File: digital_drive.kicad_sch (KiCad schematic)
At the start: 19 parts, among them U1501 EPC23104ENGRT, U1502 EPC23104ENGRT

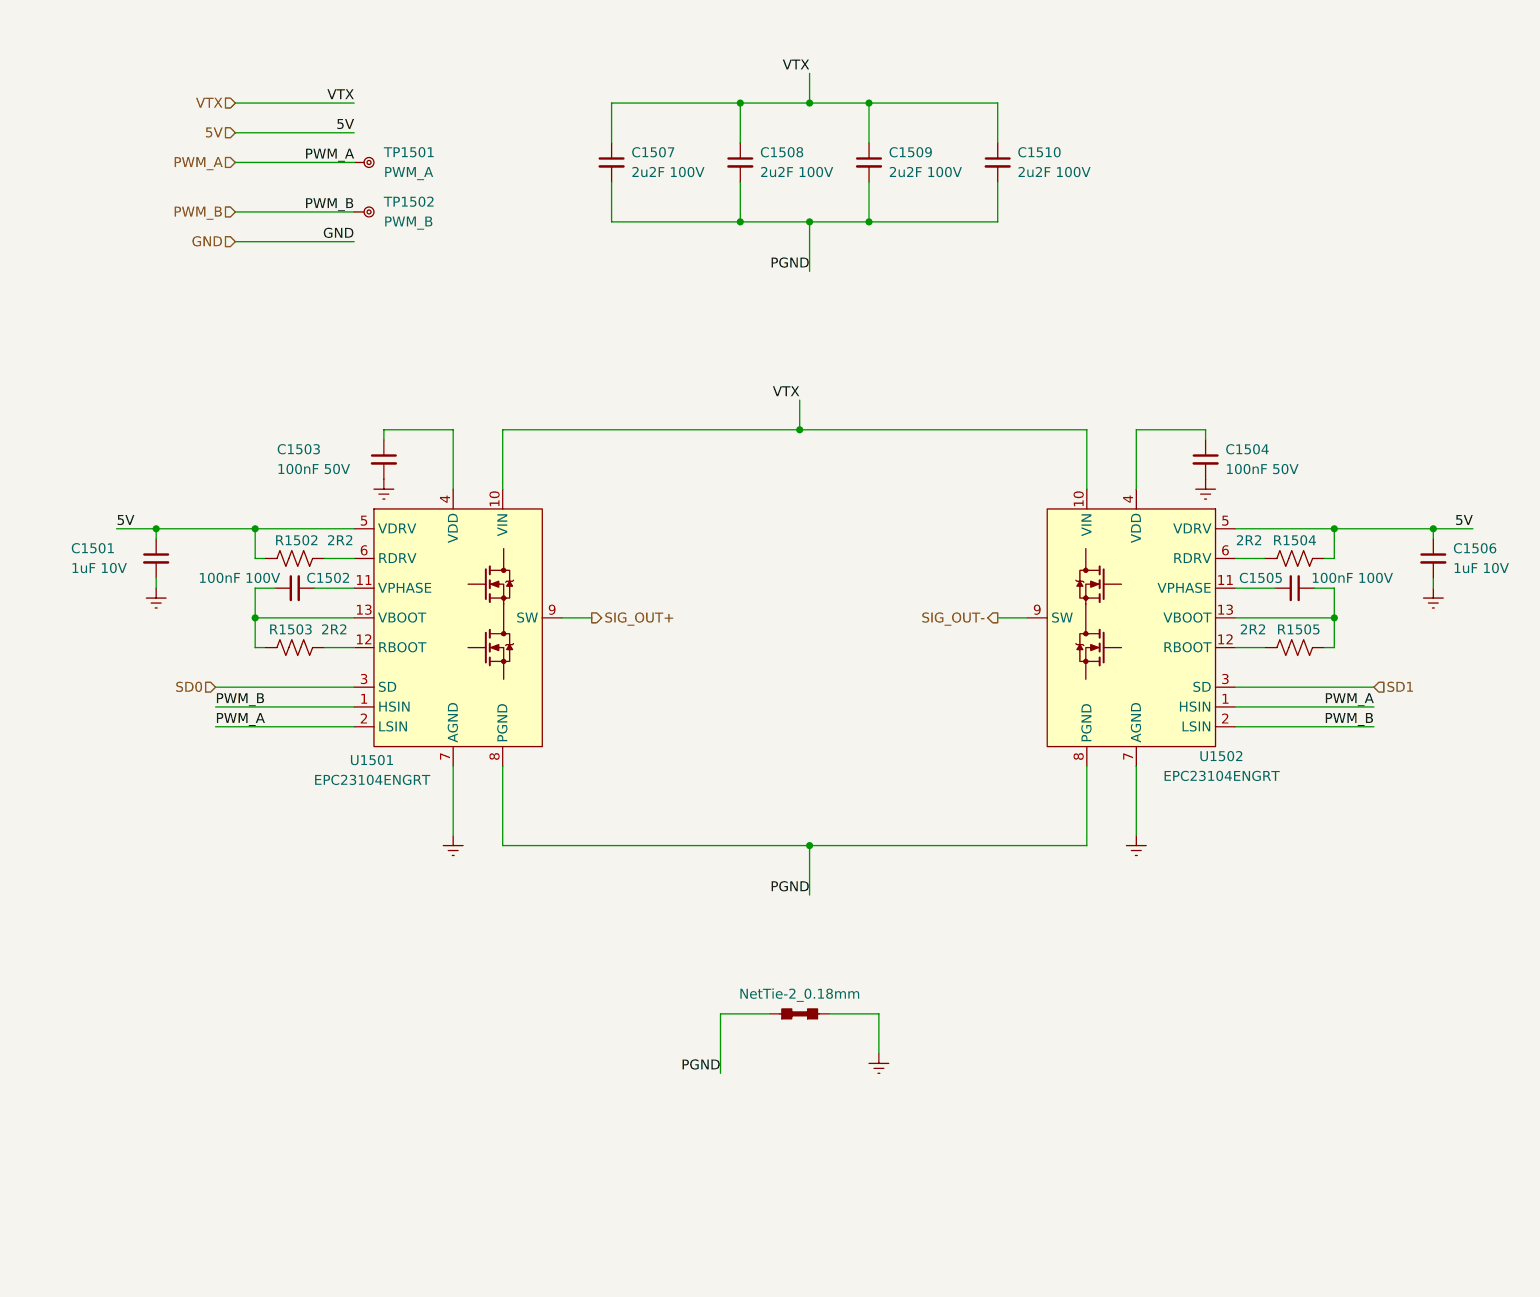
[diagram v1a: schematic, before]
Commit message: more work
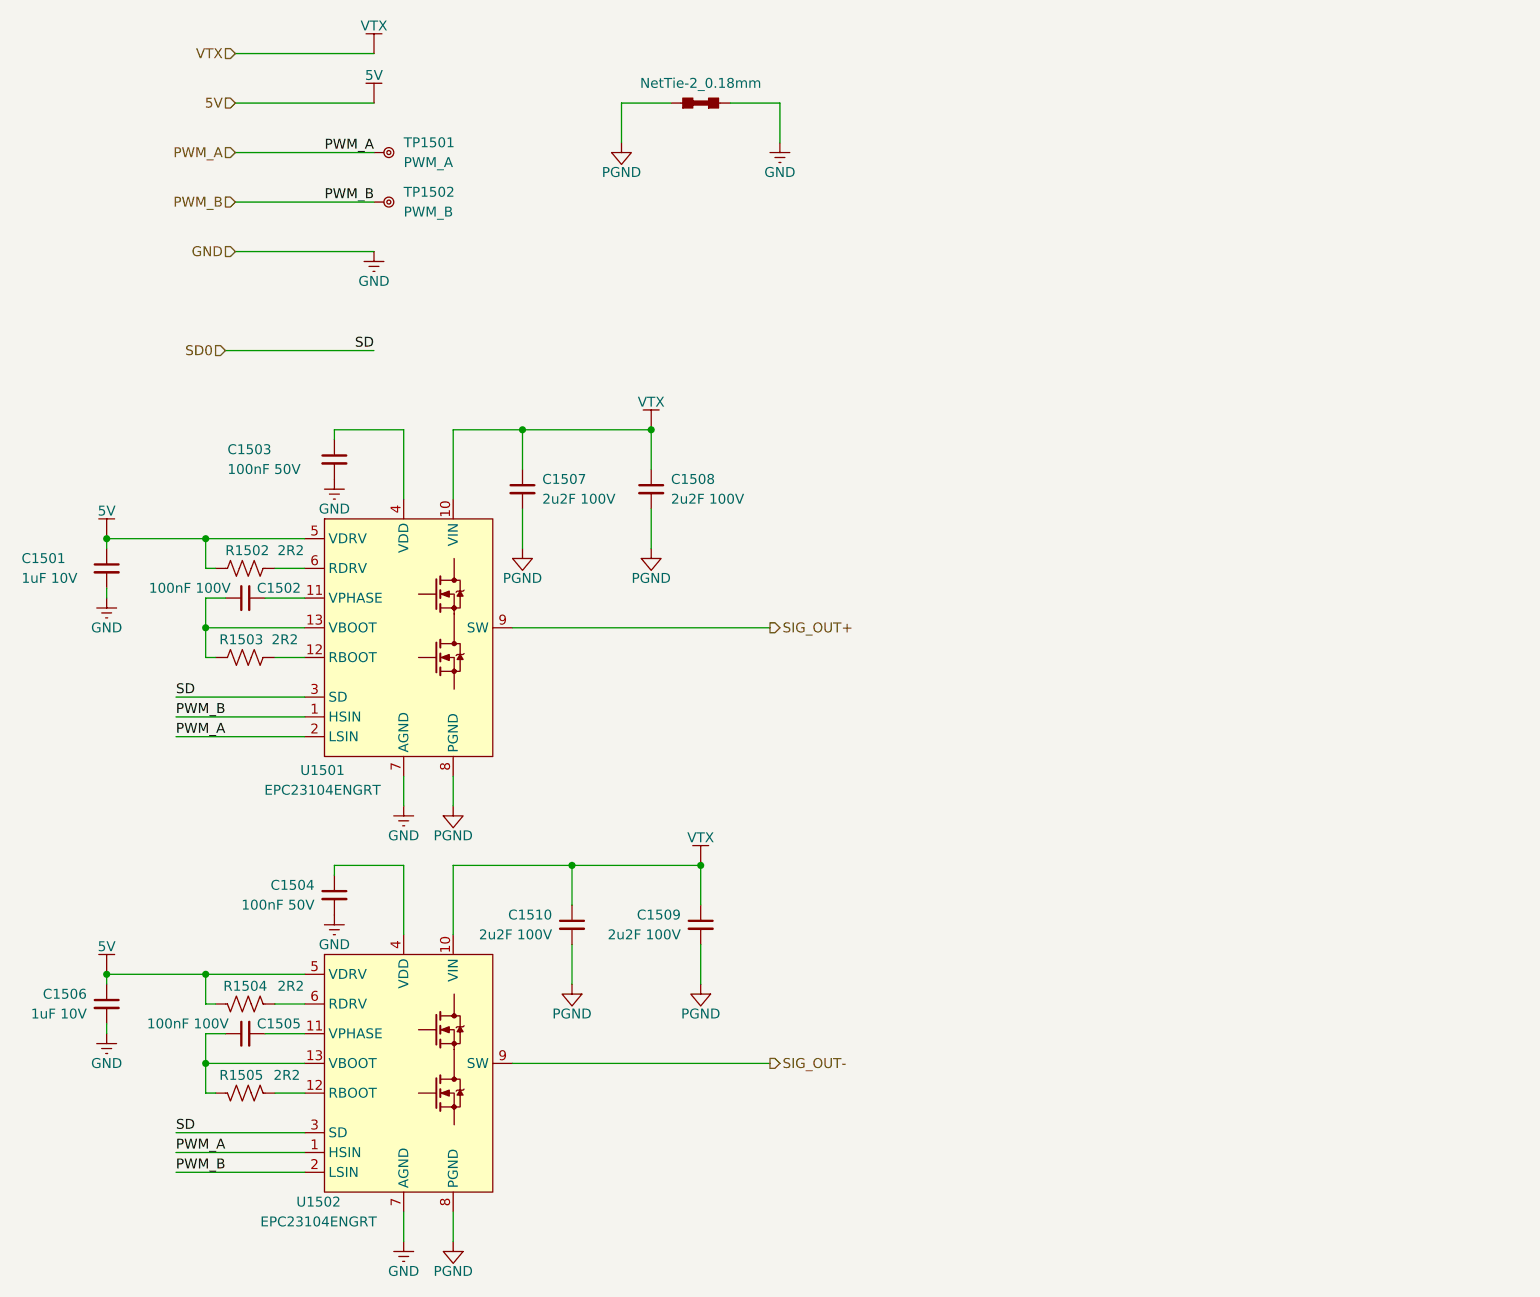
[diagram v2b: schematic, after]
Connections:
- net SD1 is gone; now on net SD0: U1502.3 (SD)
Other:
- moved on the sheet: C1501, C1502, C1503, C1504, C1505, C1506, C1507, C1508, C1509, C1510, R1502, R1503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
